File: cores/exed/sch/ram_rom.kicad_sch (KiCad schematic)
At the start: 8 parts

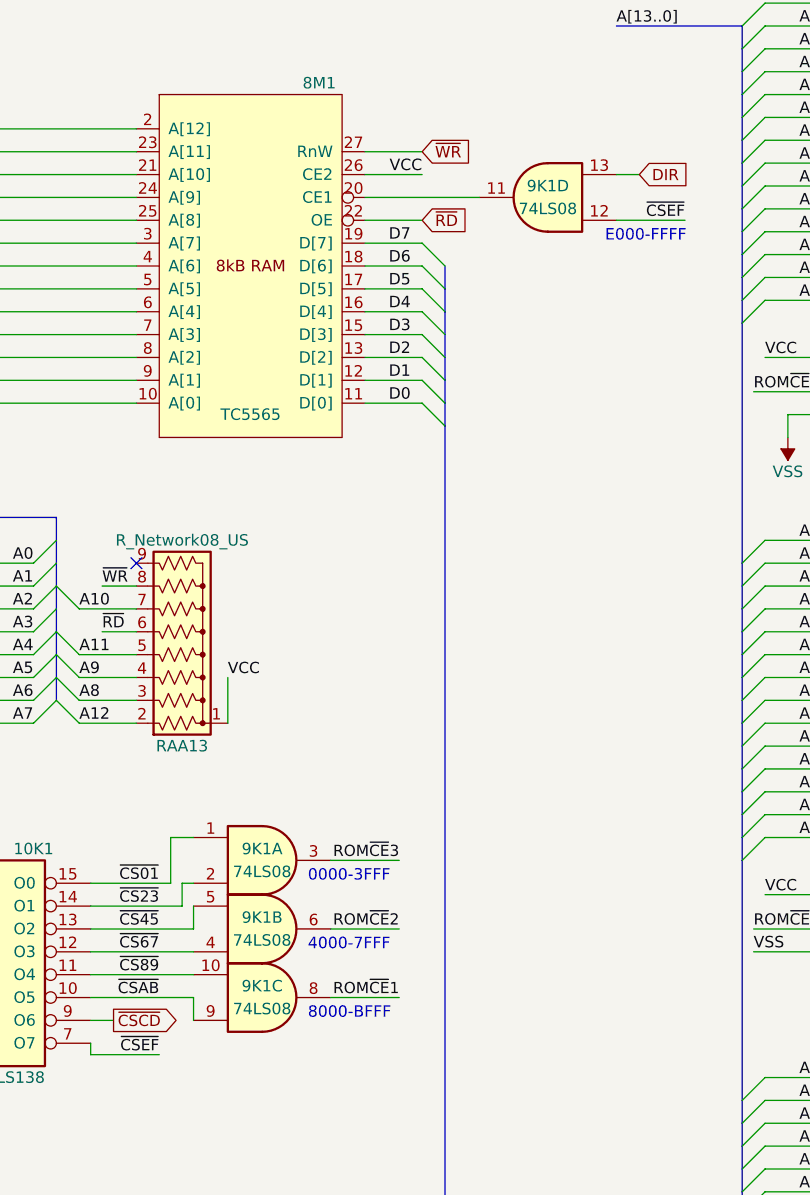
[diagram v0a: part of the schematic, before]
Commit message: issue #577 #578
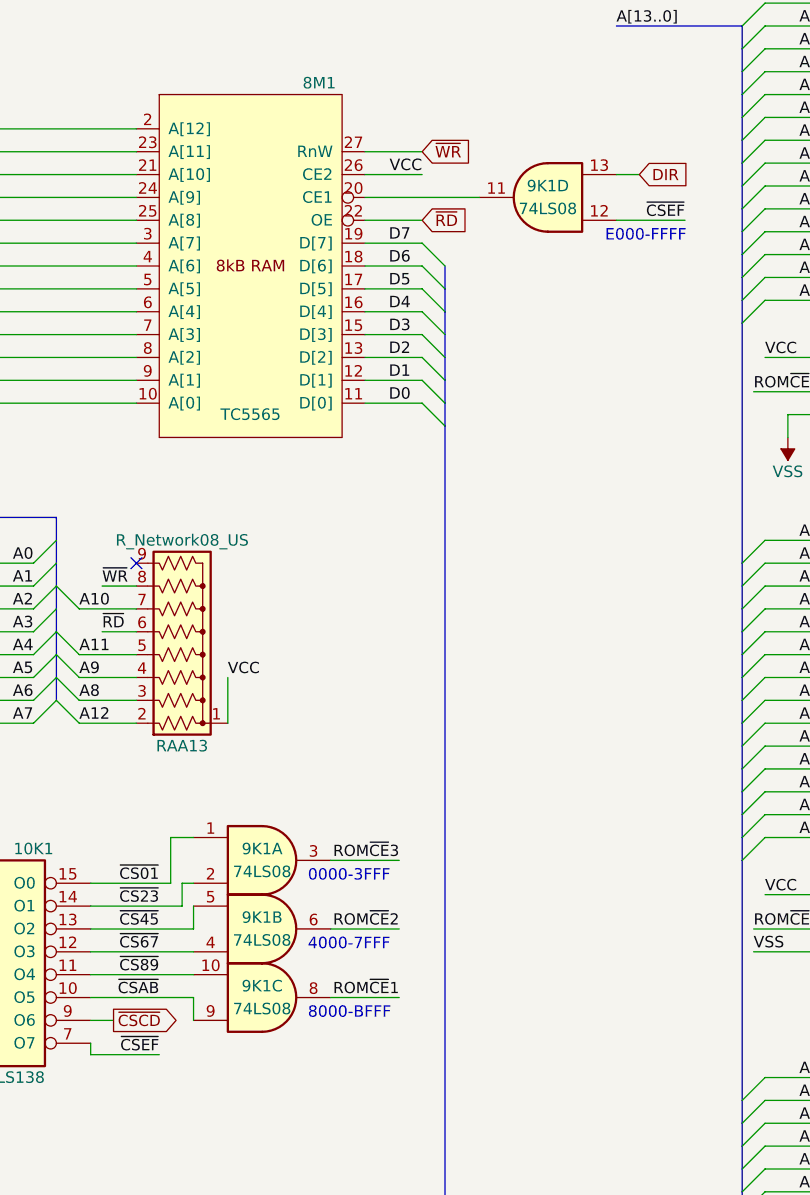
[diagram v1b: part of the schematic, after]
